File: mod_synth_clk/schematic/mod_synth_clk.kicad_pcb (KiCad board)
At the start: 2 copper layers, 17.8 x 109.2 mm, 9 parts, among them J1 Clock, J2 Conn_02x08_Odd_Even

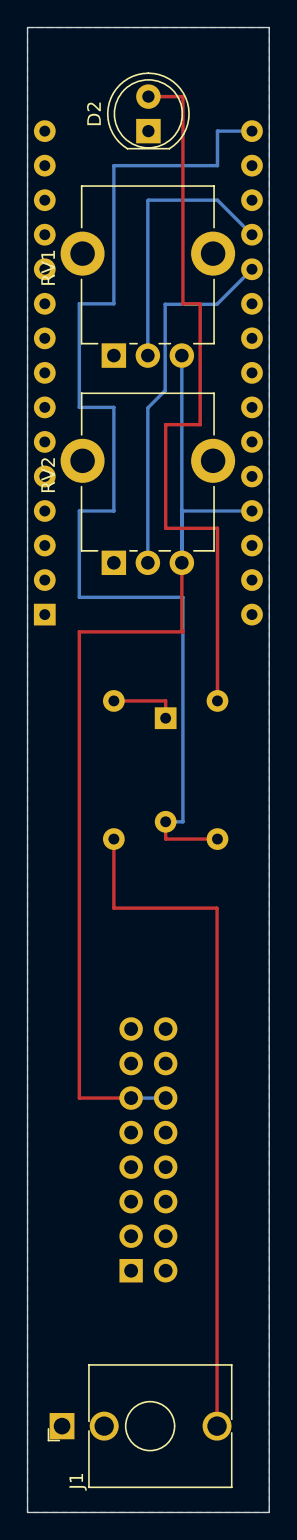
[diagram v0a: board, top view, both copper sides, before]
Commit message: Update PCB layouts
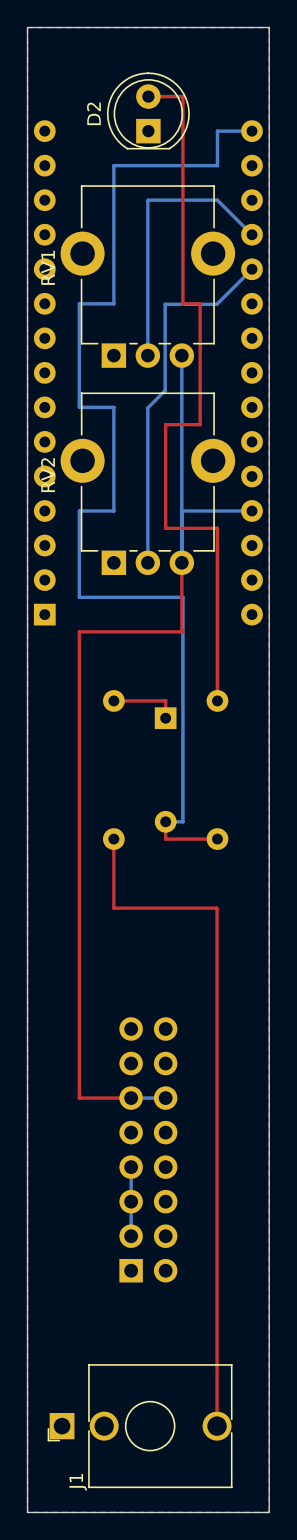
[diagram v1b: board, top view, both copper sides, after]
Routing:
- net Net-(J2-Pad3): track 0.00 -> 5.08 mm
- added copper zone on F.Cu, net GND
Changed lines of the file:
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@@
     (thickness 1.6)
     (drawings 4)
-    (tracks 49)
+    (tracks 51)
     (zones 0)
     (modules 9)
@@
   (segment (start 52.04 90.2) (end 52.04 128.27) (width 0.25) (layer F.Cu) (net 33))
   (segment (start 52.01 90.17) (end 52.04 90.2) (width 0.25) (layer F.Cu) (net 33))
+  (segment (start 45.72 109.22) (end 45.72 111.76) (width 0.25) (layer B.Cu) (net 40))
+  (segment (start 45.72 114.3) (end 45.72 111.76) (width 0.25) (layer B.Cu) (net 40))
+  (zone (net 5) (net_name GND) (layer F.Cu) (hatch edge 0.508)
+    (connect_pads (clearance 0.508))
+    (min_thickness 0.254)
+    (fill yes (arc_segments 32) (thermal_gap 0.508) (thermal_bridge_width 0.508))
+    (polygon
+      (pts
+        (xy 38.1 25.4) (xy 55.88 25.4) (xy 55.88 134.62) (xy 38.1 134.62)
+      )
+    )
+  )
   (zone (net 5) (net_name GND) (layer B.Cu) (hatch edge 0.508)
     (connect_pads (clearance 0.508))
@@
     (polygon
       (pts
-        (xy 55.88 134.62) (xy 38.1 134.62) (xy 38.1 25.4) (xy 55.88 25.4)
+        (xy 38.1 25.4) (xy 55.88 25.4) (xy 55.88 134.62) (xy 38.1 134.62)
       )
     )
